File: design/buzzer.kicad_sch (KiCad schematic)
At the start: 3 parts, among them J1 Conn_01x04_Pin, U6 ATtiny84A-M

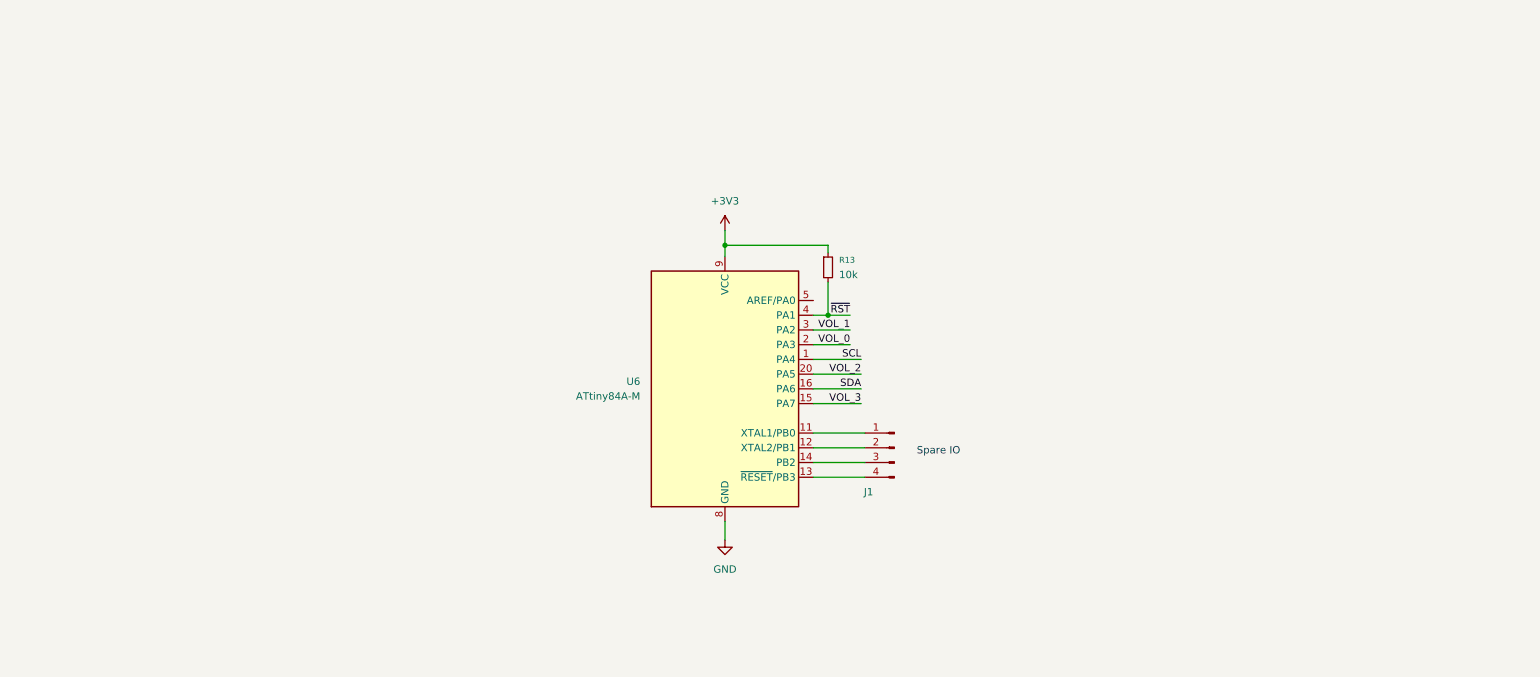
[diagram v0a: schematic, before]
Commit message: layout mostly done, schematic is done, need to generate new updated pdf
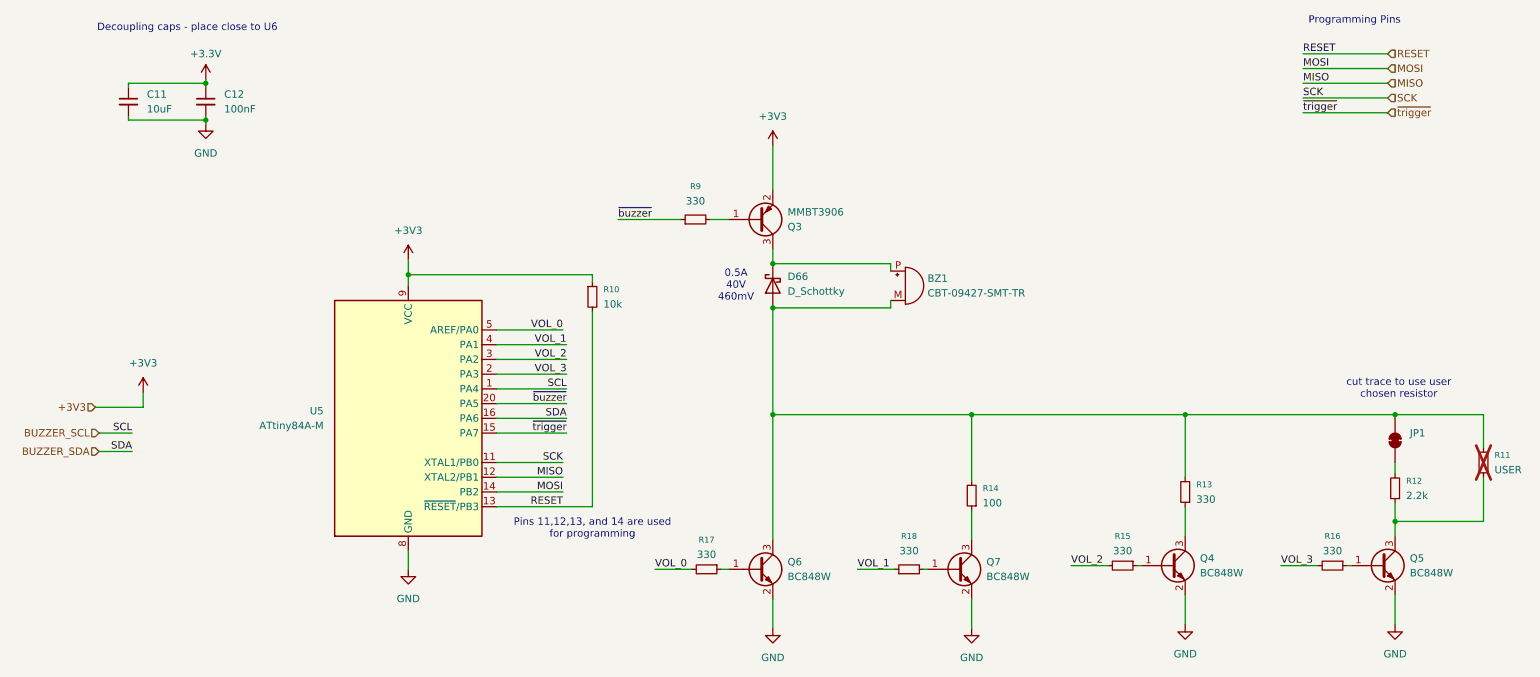
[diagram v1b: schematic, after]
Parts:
- removed J1: Conn_01x04_Pin, symbol Connector:Conn_01x04_Pin
- added BZ1: CBT-09427-SMT-TR, footprints:CUI_CBT-09427-SMT, symbol Device:Buzzer
- added C11: 10uF, Capacitor_SMD:C_0402_1005Metric_Pad0.74x0.62mm_HandSolder, symbol Device:C_Small
- added C12: 100nF, Capacitor_SMD:C_0402_1005Metric_Pad0.74x0.62mm_HandSolder, symbol Device:C_Small
- added D66: D_Schottky, Diode_SMD:D_SOD-123, symbol Device:D_Schottky
- added JP1: SolderJumper_2_Bridged, Jumper:SolderJumper-2_P1.3mm_Bridged2Bar_RoundedPad1.0x1.5mm, symbol Jumper:SolderJumper_2_Bridged
- added Q3: MMBT3906, Package_TO_SOT_SMD:SOT-23, symbol Transistor_BJT:MMBT3906
- added Q4, Q5, Q6, Q7: BC848W, Package_TO_SOT_SMD:SOT-323_SC-70, symbol Transistor_BJT:BC848W
- added R11: USER, Resistor_SMD:R_0402_1005Metric_Pad0.72x0.64mm_HandSolder, symbol Device:R_Small
- added R12: 2.2k, Resistor_SMD:R_0402_1005Metric_Pad0.72x0.64mm_HandSolder, symbol Device:R_Small
- added R13, R15, R16, R17, R18, R9: 330, Resistor_SMD:R_0402_1005Metric_Pad0.72x0.64mm_HandSolder, symbol Device:R_Small
- added R14: 100, Resistor_SMD:R_0402_1005Metric_Pad0.72x0.64mm_HandSolder, symbol Device:R_Small
- renumbered R13 to R10, U6 to U5
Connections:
- net +3V3: now also Q3.2 (E)
- net GND: now also C11.2, C12.2, Q4.2 (E), Q5.2 (E), Q6.2 (E), Q7.2 (E)
- net VOL_0: now also U5.5 (AREF/PA0), R17.2; no longer U5.2 (PA3)
- net VOL_1: now also U5.4 (PA1), R18.1; no longer U5.3 (PA2)
- net VOL_2: now also U5.3 (PA2), R15.2; no longer U5.20 (PA5)
- net VOL_3: now also U5.2 (PA3), R16.2; no longer U5.15 (PA7)
- net SCK: now reaches U5.11 (XTAL1/PB0)
- net MISO: now reaches U5.12 (XTAL2/PB1)
- net MOSI: now reaches U5.14 (PB2)
- net RESET: now reaches U5.13 (~{RESET}/PB3)
- net RESET: now also R10.2
- net SCL renamed BUZZER_SCL
- net SDA renamed BUZZER_SDA
- removed net ~{RST}: R10.2, U5.4 (PA1)
- new net: Q5.1 (B), R16.1
- new net: Q5.3 (C), R11.1, R12.1
- new net: Q6.1 (B), R17.1
- new net: BZ1.M, D66.2 (A), JP1.2 (B), Q6.3 (C), R11.2, R13.2, R14.2
- new net: Q3.1 (B), R9.2
- new net: BZ1.P, D66.1 (K), Q3.3 (C)
- new net: Q4.1 (B), R15.1
- new net: Q7.1 (B), R18.2
- new net: Q4.3 (C), R13.1
- new net: Q7.3 (C), R14.1
- new net: JP1.1 (A), R12.2
- new net +3.3V: C11.1, C12.1
- new net ~{buzzer}: R9.1, U5.20 (PA5)
- new net ~{trigger}: U5.15 (PA7)
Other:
- note added: "0.5A 40V 460mV"
- note added: "Decoupling caps - place close to U6"
- note added: "Pins 11,12,13, and 14 are used for programming"
- note added: "Programming Pins"
- note added: "cut trace to use user chosen resistor"
- note removed: "Spare IO"
- moved on the sheet: R10, U5
